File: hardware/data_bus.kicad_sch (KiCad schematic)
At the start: 11 parts, among them Q13 BC547, U10 74HC595, U11 74HC165, U12 74HC165, U9 74HC595

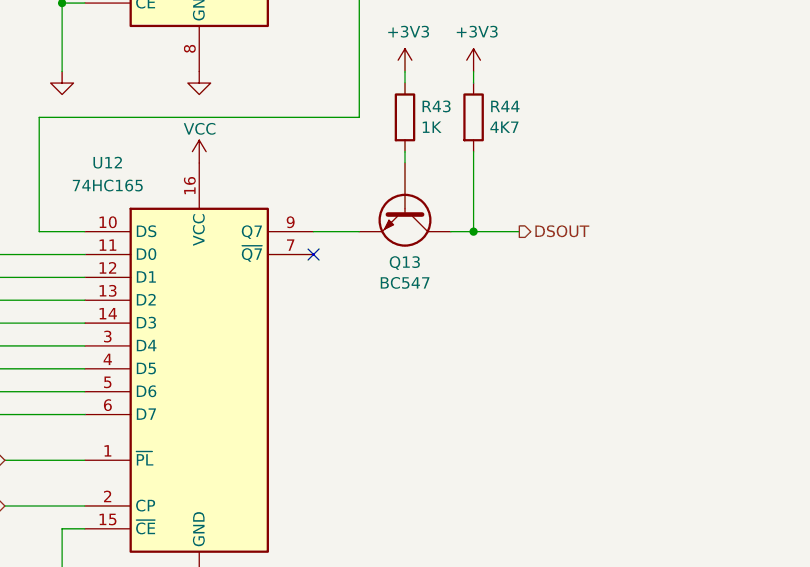
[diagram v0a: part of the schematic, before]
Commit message: Rev.E. Updated specifications document and hardware design.
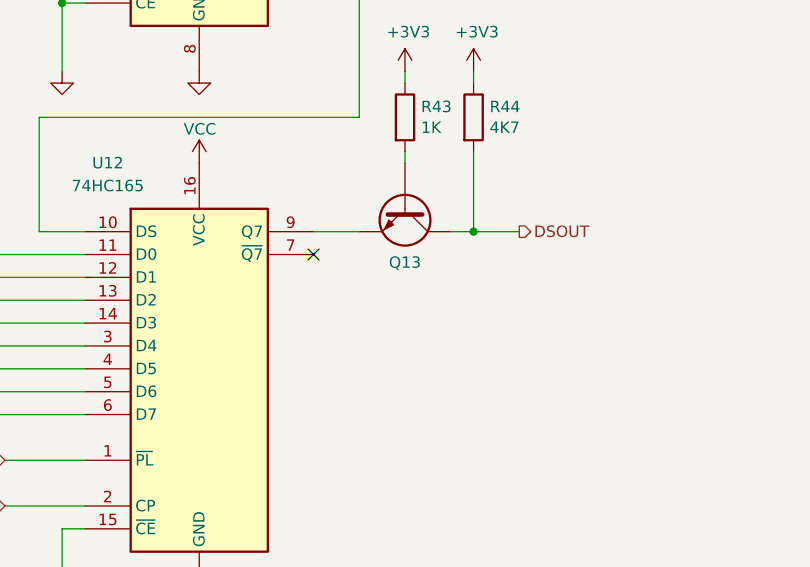
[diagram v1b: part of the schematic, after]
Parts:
- Q13: value BC547 -> (none); footprint Package_TO_SOT_THT:TO-92_Inline_Wide -> (none)
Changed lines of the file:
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@@
     (in_bom yes) (on_board yes)
     (property "Reference" "Q13" (id 0) (at 76.2 91.059 90))
-    (property "Value" "BC547" (id 1) (at 76.2 93.3704 90))
-    (property "Footprint" "Package_TO_SOT_THT:TO-92_Inline_Wide" (id 2) (at 74.295 90.17 0)
+    (property "Value" "" (id 1) (at 76.2 93.3704 90))
+    (property "Footprint" "" (id 2) (at 74.295 90.17 0)
       (effects (font (size 1.27 1.27) italic) (justify left) hide)
     )
